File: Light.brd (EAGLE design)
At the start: 20.3 x 25.1 mm, 3 parts, among them X1 IR

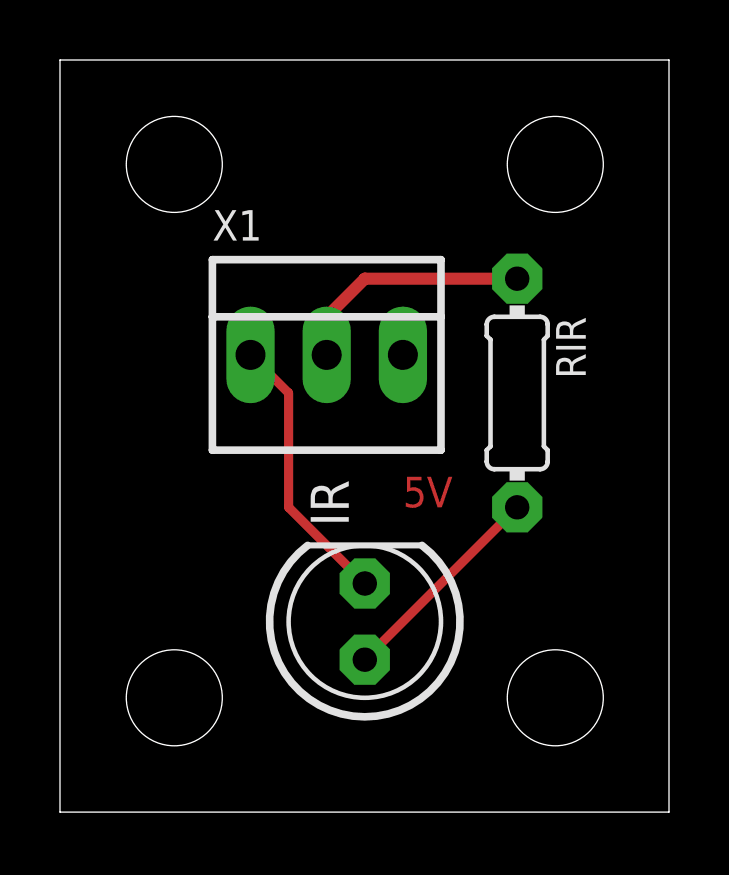
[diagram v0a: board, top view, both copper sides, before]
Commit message: 29/10/2013
Fixed:
-Naming in PIN
-PIR & Light Sensor PCB
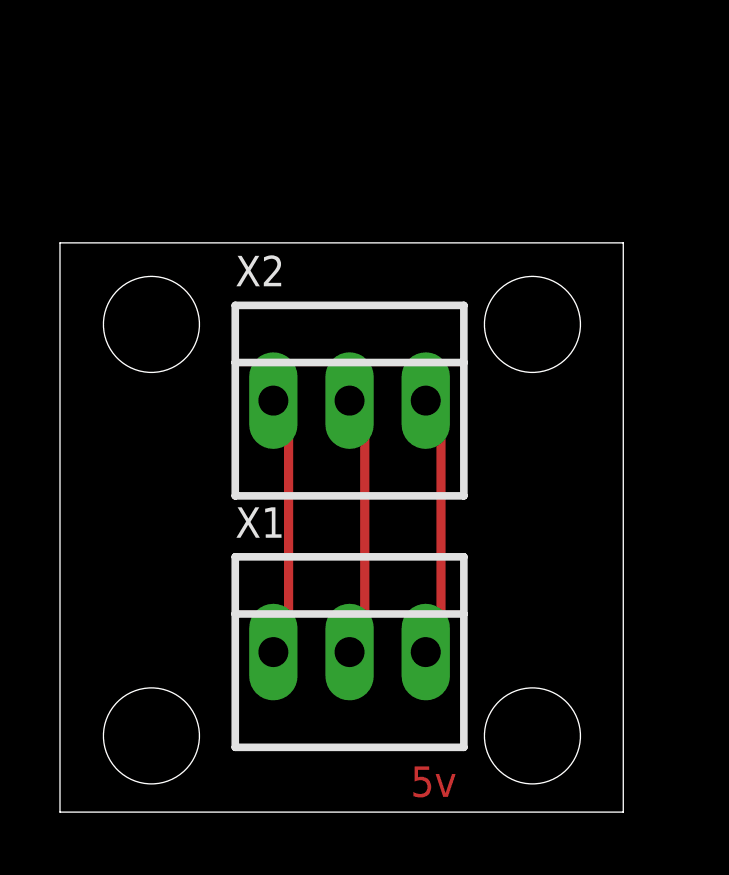
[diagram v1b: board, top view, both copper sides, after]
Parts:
- removed IR: (no value), adafruit:LED5MM
- removed RIR: 220, adafruit:0204/7
- added X2: LIGHT, con-molex:22-23-2031
- X1: value IR -> SIGNAL
- moved X1 9.94 mm to (9.65, 5.33)
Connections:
- removed net N$2: RIR.1, X1.2
- removed net N$4: IR.A, RIR.2
- new net SIG: X1.2, X2.2
- net +5V: now also X2.3
- net GND: now also X2.1; no longer IR.K
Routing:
- net SIG: track 0.00 -> 8.62 mm
- net +5V: track 0.00 -> 8.62 mm
- net N$2: track 8.15 -> 0.00 mm
- net N$4: track 7.18 -> 0.00 mm
- net GND: track 9.20 -> 8.62 mm
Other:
- board size 20.3 x 25.1 mm -> 18.8 x 19 mm
- board text added: "5v"
- board text removed: "5V"
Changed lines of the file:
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@@
 <setting verticaltext="up"/>
 </settings>
-<grid distance="0.05" unitdist="inch" unit="inch" style="lines" multiple="1" display="yes" altdistance="0.025" altunitdist="inch" altunit="inch"/>
+<grid distance="0.02" unitdist="inch" unit="inch" style="lines" multiple="1" display="yes" altdistance="0.025" altunitdist="inch" altunit="inch"/>
 <layers>
 <layer number="1" name="Top" color="4" fill="1" visible="yes" active="yes"/>
@@
 <board>
 <plain>
-<wire x1="0" y1="0" x2="20.3" y2="0" width="0" layer="20"/>
-<wire x1="20.3" y1="0" x2="20.3" y2="25.07" width="0" layer="20"/>
-<wire x1="20.3" y1="25.07" x2="0" y2="25.07" width="0" layer="20"/>
-<wire x1="0" y1="25.07" x2="0" y2="0" width="0" layer="20"/>
-<hole x="16.51" y="3.81" drill="3.2"/>
-<hole x="3.81" y="3.81" drill="3.2"/>
-<hole x="3.81" y="21.59" drill="3.2"/>
-<hole x="16.51" y="21.59" drill="3.2"/>
-<text x="11.43" y="10.16" size="1.016" layer="1">5V</text>
+<wire x1="0" y1="0" x2="18.776" y2="0" width="0" layer="20"/>
+<wire x1="18.776" y1="0" x2="18.776" y2="18.974" width="0" layer="20"/>
+<wire x1="18.776" y1="18.974" x2="0" y2="18.974" width="0" layer="20"/>
+<wire x1="0" y1="18.974" x2="0" y2="0" width="0" layer="20"/>
+<hole x="3.048" y="16.256" drill="3.2"/>
+<hole x="3.048" y="2.54" drill="3.2"/>
+<hole x="15.748" y="16.256" drill="3.2"/>
+<hole x="15.748" y="2.54" drill="3.2"/>
+<text x="11.684" y="0.508" size="1.016" layer="1">5v</text>
 </plain>
 <attributes>
@@
 </variantdefs>
 <classes>
-<class number="0" name="default" width="0" drill="0">
+<class number="0" name="default" width="0.254" drill="0">
+<clearance class="0" value="0.254"/>
 </class>
 </classes>
@@
 </autorouter>
 <elements>
-<element name="X1" library="con-molex" package="22-23-2031" value="IR" x="8.89" y="15.24">
-<attribute name="OC_NEWARK" value="30C0862" x="26.67" y="8.89" size="1.778" layer="27" display="off"/>
-<attribute name="MPN" value="22-23-2031" x="26.67" y="8.89" size="1.778" layer="27" display="off"/>
-<attribute name="MF" value="MOLEX" x="26.67" y="8.89" size="1.778" layer="27" display="off"/>
-<attribute name="OC_FARNELL" value="1462950" x="26.67" y="8.89" size="1.778" layer="27" display="off"/>
+<element name="X1" library="con-molex" package="22-23-2031" value="SIGNAL" x="9.652" y="5.334">
+<attribute name="OC_NEWARK" value="30C0862" x="27.432" y="-1.016" size="1.778" layer="27" display="off"/>
+<attribute name="MPN" value="22-23-2031" x="27.432" y="-1.016" size="1.778" layer="27" display="off"/>
+<attribute name="MF" value="MOLEX" x="27.432" y="-1.016" size="1.778" layer="27" display="off"/>
+<attribute name="OC_FARNELL" value="1462950" x="27.432" y="-1.016" size="1.778" layer="27" display="off"/>
 </element>
-<element name="RIR" library="adafruit" package="0204/7" value="220" x="15.24" y="13.97" rot="R270"/>
-<element name="IR" library="adafruit" package="LED5MM" value="" x="10.16" y="6.35" rot="R90"/>
+<element name="X2" library="con-molex" package="22-23-2031" value="LIGHT" x="9.652" y="13.716">
+<attribute name="OC_NEWARK" value="30C0862" x="27.432" y="-4.064" size="1.778" layer="27" display="off"/>
+<attribute name="MPN" value="22-23-2031" x="27.432" y="-4.064" size="1.778" layer="27" display="off"/>
+<attribute name="MF" value="MOLEX" x="27.432" y="-4.064" size="1.778" layer="27" display="off"/>
+<attribute name="OC_FARNELL" value="1462950" x="27.432" y="-4.064" size="1.778" layer="27" display="off"/>
+</element>
 </elements>
 <signals>
-<signal name="N$2">
-<contactref element="X1" pad="2"/>
-<contactref element="RIR" pad="1"/>
-<wire x1="8.89" y1="15.24" x2="8.89" y2="16.51" width="0.4064" layer="1"/>
-<wire x1="8.89" y1="16.51" x2="10.16" y2="17.78" width="0.4064" layer="1"/>
-<wire x1="10.16" y1="17.78" x2="15.24" y2="17.78" width="0.4064" layer="1"/>
-</signal>
-<signal name="N$4">
-<contactref element="RIR" pad="2"/>
-<contactref element="IR" pad="A"/>
-<wire x1="15.24" y1="10.16" x2="10.16" y2="5.08" width="0.3048" layer="1"/>
-</signal>
 <signal name="GND">
 <contactref element="X1" pad="1"/>
-<contactref element="IR" pad="K"/>
-<wire x1="7.62" y1="13.97" x2="6.35" y2="15.24" width="0.3048" layer="1"/>
-<wire x1="7.62" y1="10.16" x2="7.62" y2="13.97" width="0.3048" layer="1"/>
-<wire x1="10.16" y1="7.62" x2="7.62" y2="10.16" width="0.3048" layer="1"/>
+<contactref element="X2" pad="1"/>
+<wire x1="7.62" y1="12.7" x2="7.62" y2="6.35" width="0.3048" layer="1"/>
+<wire x1="7.62" y1="6.35" x2="7.112" y2="5.334" width="0.3048" layer="1"/>
+<wire x1="7.62" y1="12.7" x2="7.112" y2="13.716" width="0.3048" layer="1"/>
 </signal>
 <signal name="+5V">
 <contactref element="X1" pad="3"/>
+<contactref element="X2" pad="3"/>
+<wire x1="12.7" y1="12.7" x2="12.7" y2="6.35" width="0.3048" layer="1"/>
+<wire x1="12.7" y1="6.35" x2="12.192" y2="5.334" width="0.3048" layer="1"/>
+<wire x1="12.7" y1="12.7" x2="12.192" y2="13.716" width="0.3048" layer="1"/>
+</signal>
+<signal name="SIG">
+<contactref element="X1" pad="2"/>
+<contactref element="X2" pad="2"/>
+<wire x1="10.16" y1="12.7" x2="10.16" y2="6.35" width="0.3048" layer="1"/>
+<wire x1="10.16" y1="6.35" x2="9.652" y2="5.334" width="0.3048" layer="1"/>
+<wire x1="10.16" y1="12.7" x2="9.652" y2="13.716" width="0.3048" layer="1"/>
 </signal>
 </signals>
